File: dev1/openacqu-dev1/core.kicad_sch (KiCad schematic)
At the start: 35 parts, among them J1 GSB1C41110SSHR, J2 Test Points, U1 MCP2221AT-I_ML, U2 LP5817DRLR, U3 FXL6408UMX, U4 24AA025E48T-E_OT, U5 AP2112K-3.3TRG1, U6 TPS22996HQDYCRQ1

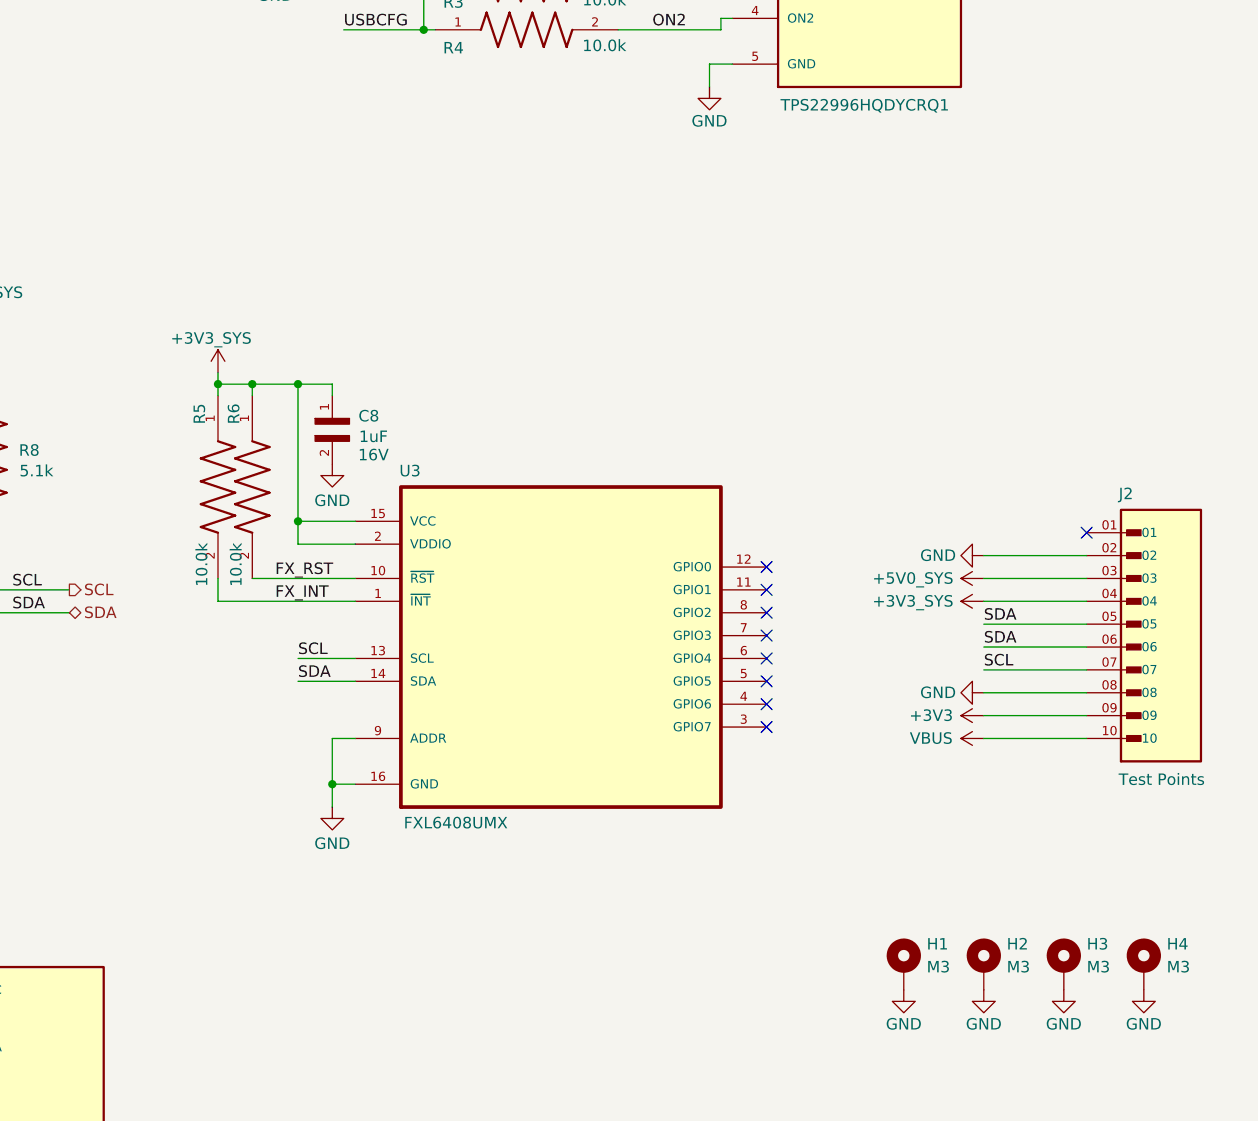
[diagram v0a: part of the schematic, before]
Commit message: Placement and routing complete for DEV1
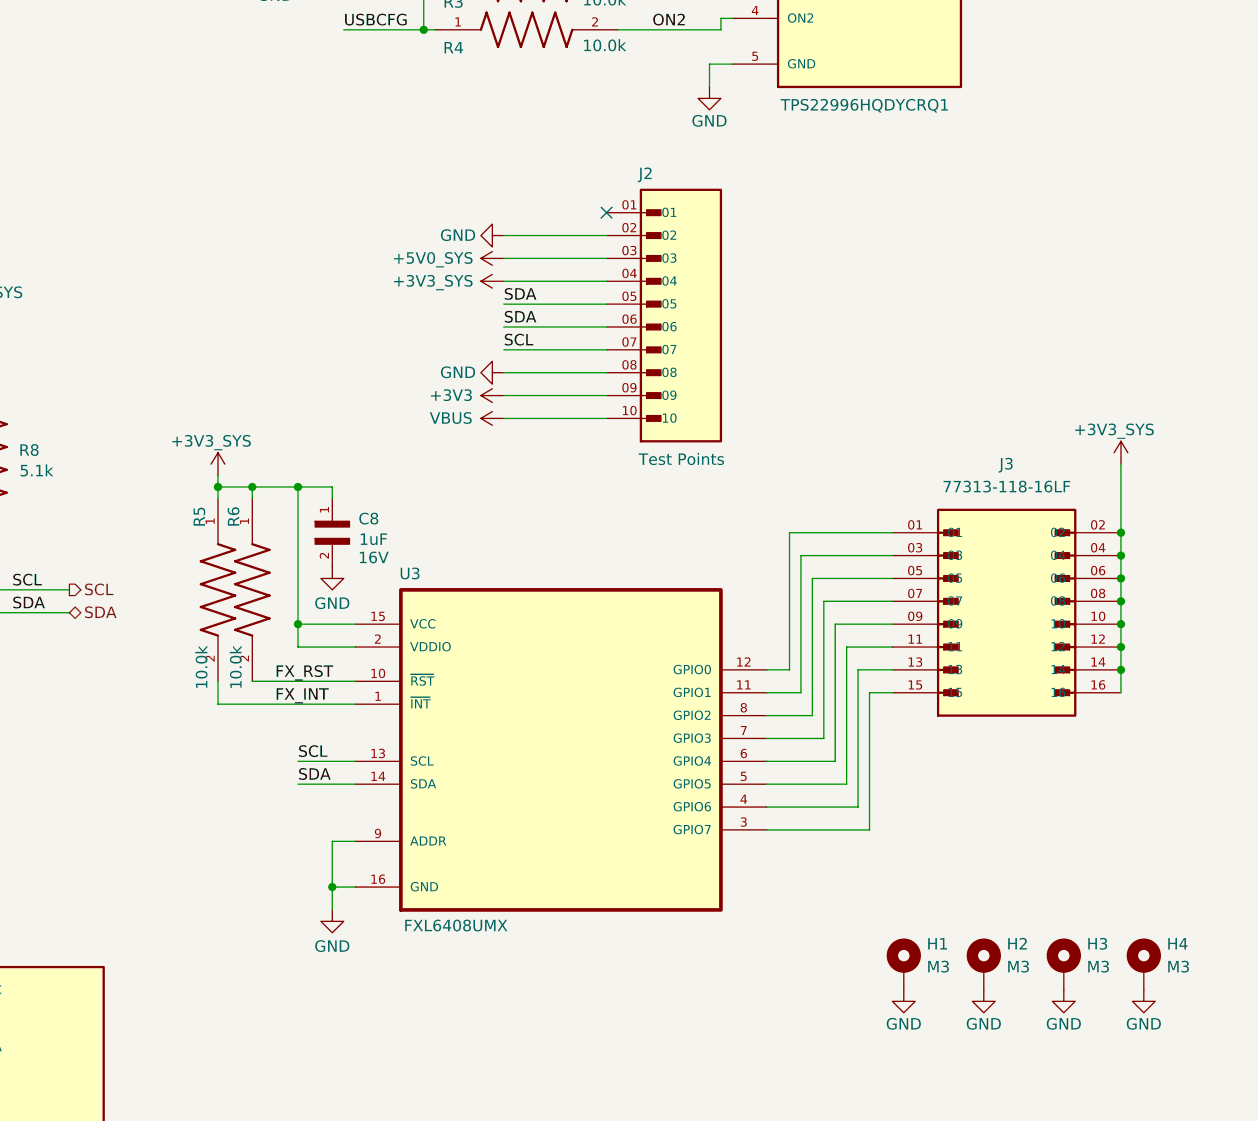
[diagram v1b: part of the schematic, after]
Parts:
- added J3: 77313-118-16LF, AMPHENOL_77313-118-16LF, symbol 77313-118-16LF:77313-118-16LF
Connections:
- net +3V3_SYS: now also J3.02, J3.04, J3.06, J3.08, J3.10, J3.12, J3.14, J3.16
- net at U3.11 (GPIO1): now also J3.03
- net at U3.12 (GPIO0): now also J3.01
- net at U3.3 (GPIO7): now also J3.15
- net at U3.4 (GPIO6): now also J3.13
- net at U3.5 (GPIO5): now also J3.11
- net at U3.6 (GPIO4): now also J3.09
- net at U3.7 (GPIO3): now also J3.07
- net at U3.8 (GPIO2): now also J3.05
- no-connect marks 19 -> 11
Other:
- moved on the sheet: C8, J2, R5, R6, U3
